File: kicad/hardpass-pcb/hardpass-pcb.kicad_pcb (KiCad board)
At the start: 2 copper layers, 30 x 65 mm, 34 parts, among them IC1 APX803, J1 Raspberry_Pi_2_3, P2 OLED_I2C, SW1 1, SW10 C/UP, SW11 0/OK, SW12 OK/DN, SW2 2, SW3 3, SW4 4, SW5 5, SW6 6, SW7 7, SW8 8, SW9 9, U2 ESP-12E

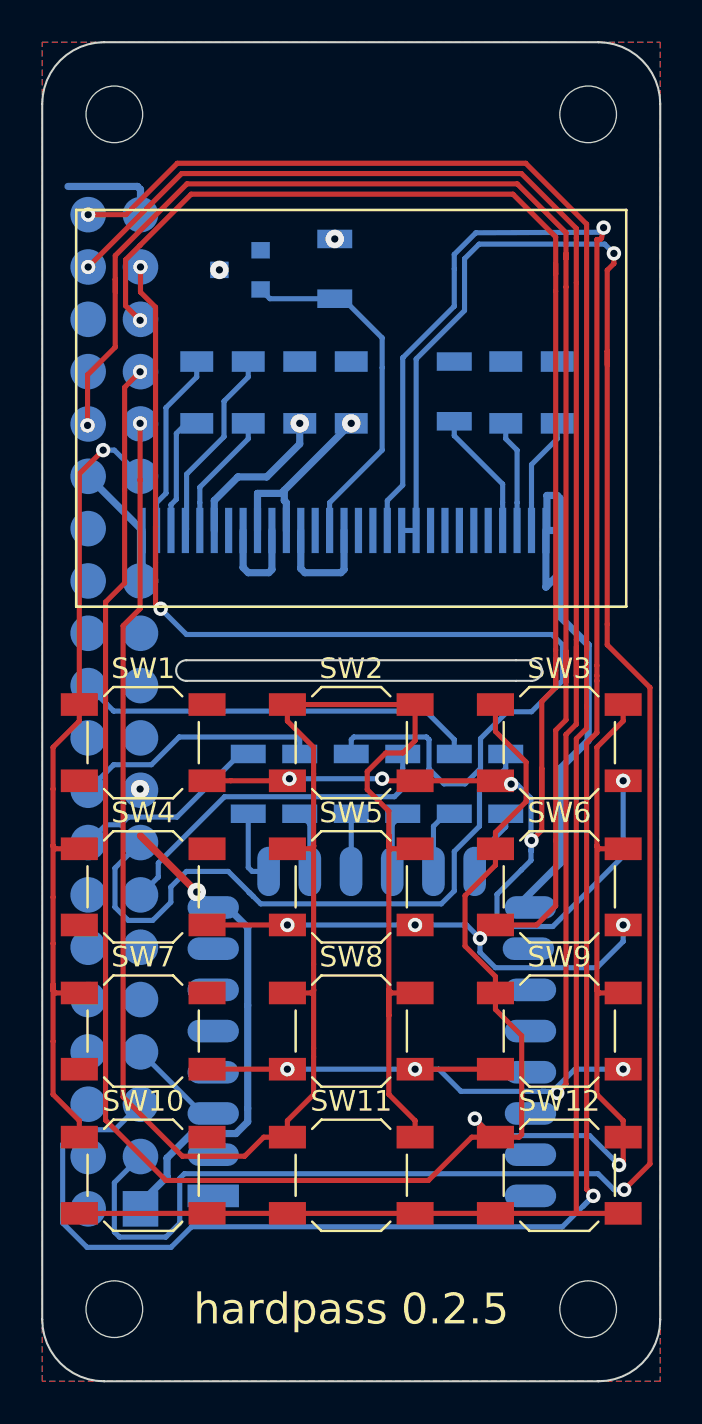
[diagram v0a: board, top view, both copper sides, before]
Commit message: cleanup on the frontend-pcb
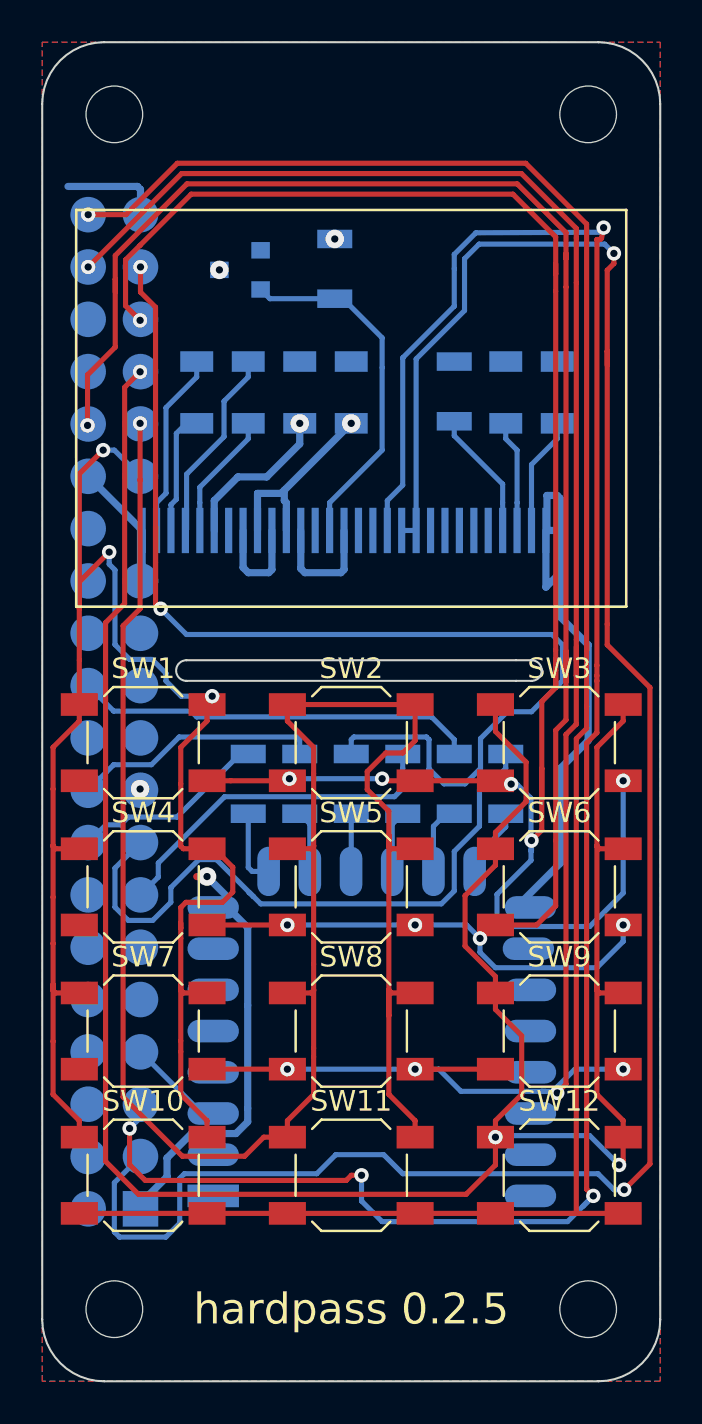
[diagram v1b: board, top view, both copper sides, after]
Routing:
- net COL_1: track 40.2 -> 82.0 mm, vias 1 -> 3
- net OLED_SCL: track 106.4 -> 99.2 mm, vias 2 -> 4
- net +3V3: track 42.4 -> 39.9 mm
- net ROW_1: track 93.8 -> 94.9 mm
- net OLED_SDA: track 102.1 -> 102.9 mm
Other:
- board text added: "Shutdown Footprint!"
